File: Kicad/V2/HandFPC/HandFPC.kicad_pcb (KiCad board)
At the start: 2 copper layers, 25 parts, among them J10 SPI_LED, J2 JST_LED_SPI_5V_GND, J3 JST_LED_SPI_5V_GND, J4 JST_LED_SPI_5V_GND, J5 JST_LED_SPI_5V_GND, J6 JST_LED_SPI_5V_GND, J7 SPI_LED, J8 SPI_LED, J9 SPI_LED, U1 ICM-42688-P_I2C, U2 Hall Sensor DRV5023

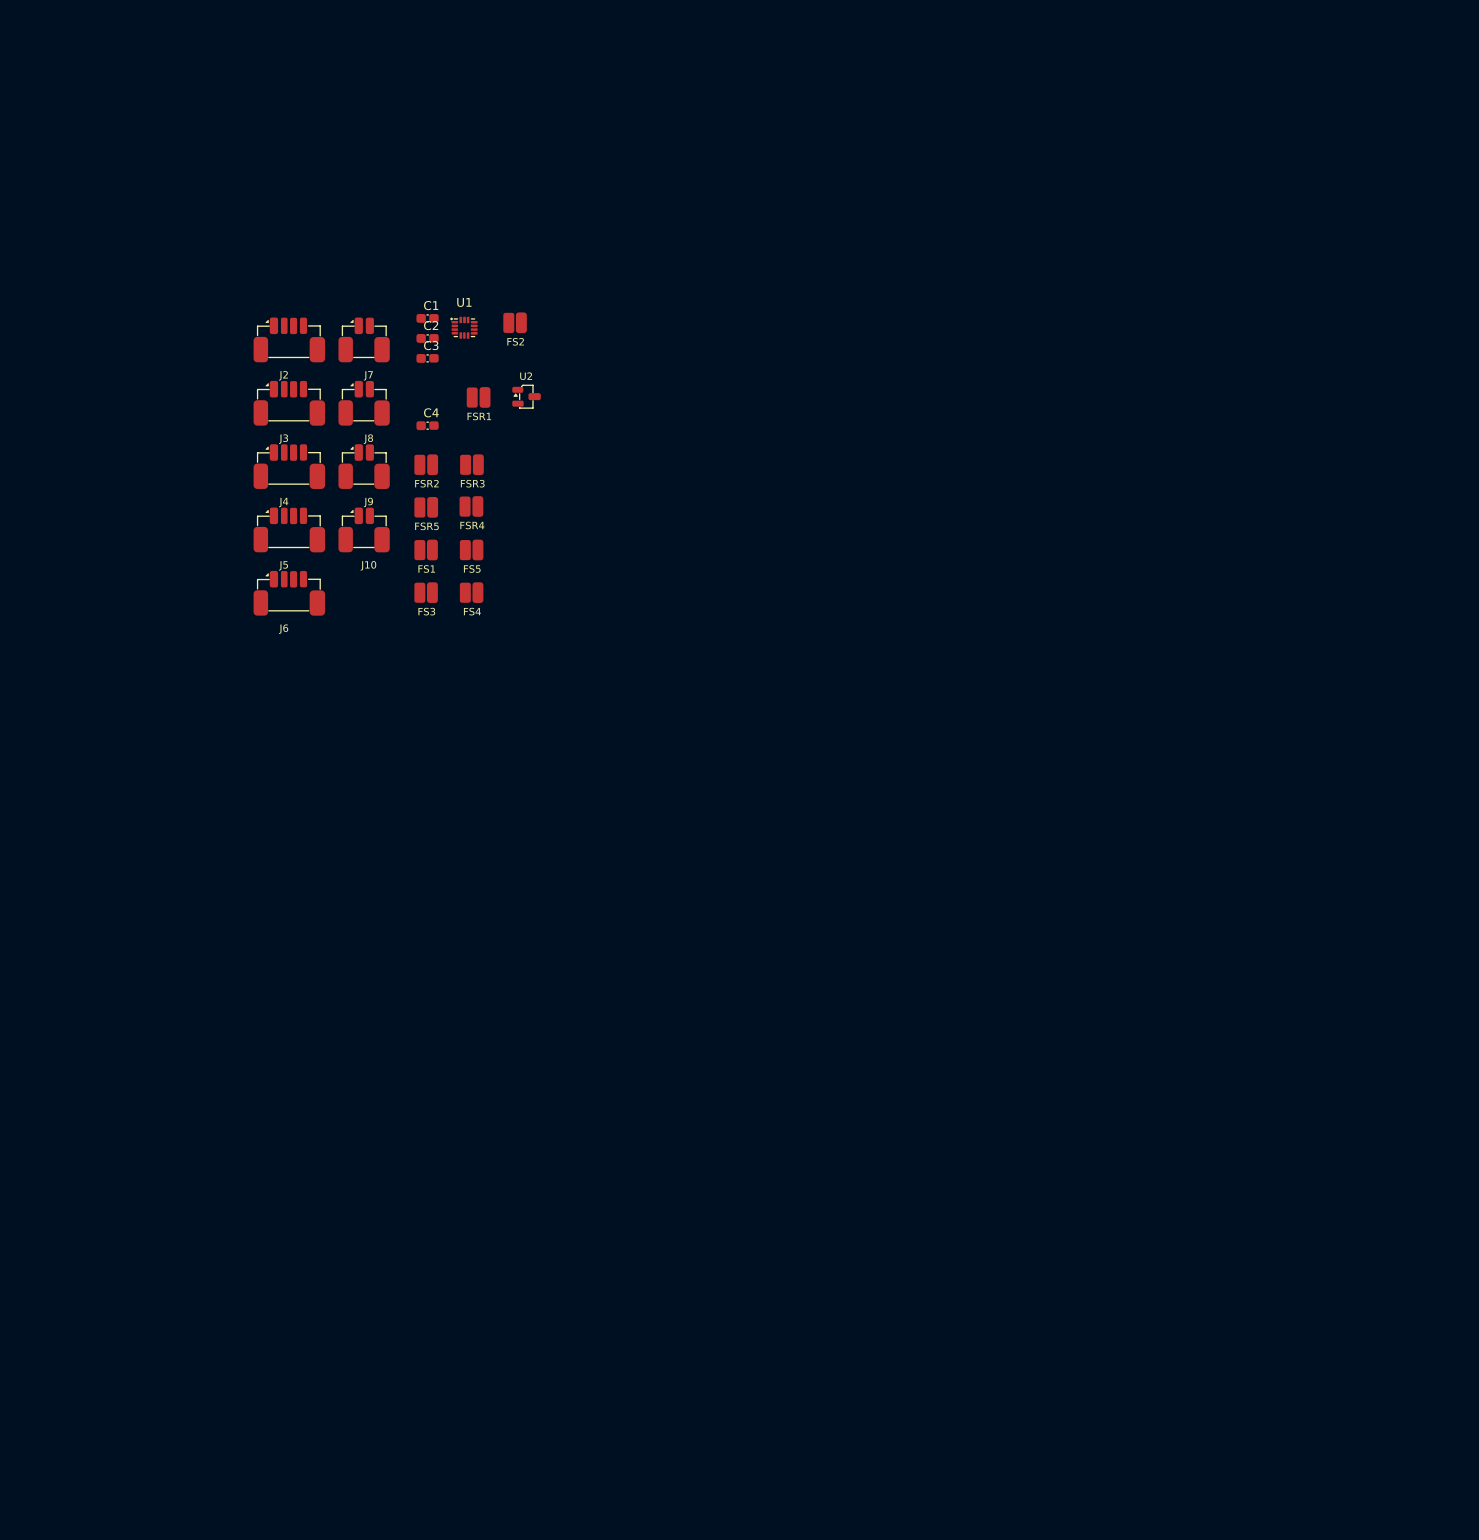
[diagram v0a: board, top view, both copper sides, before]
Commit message: add edgecut for testing
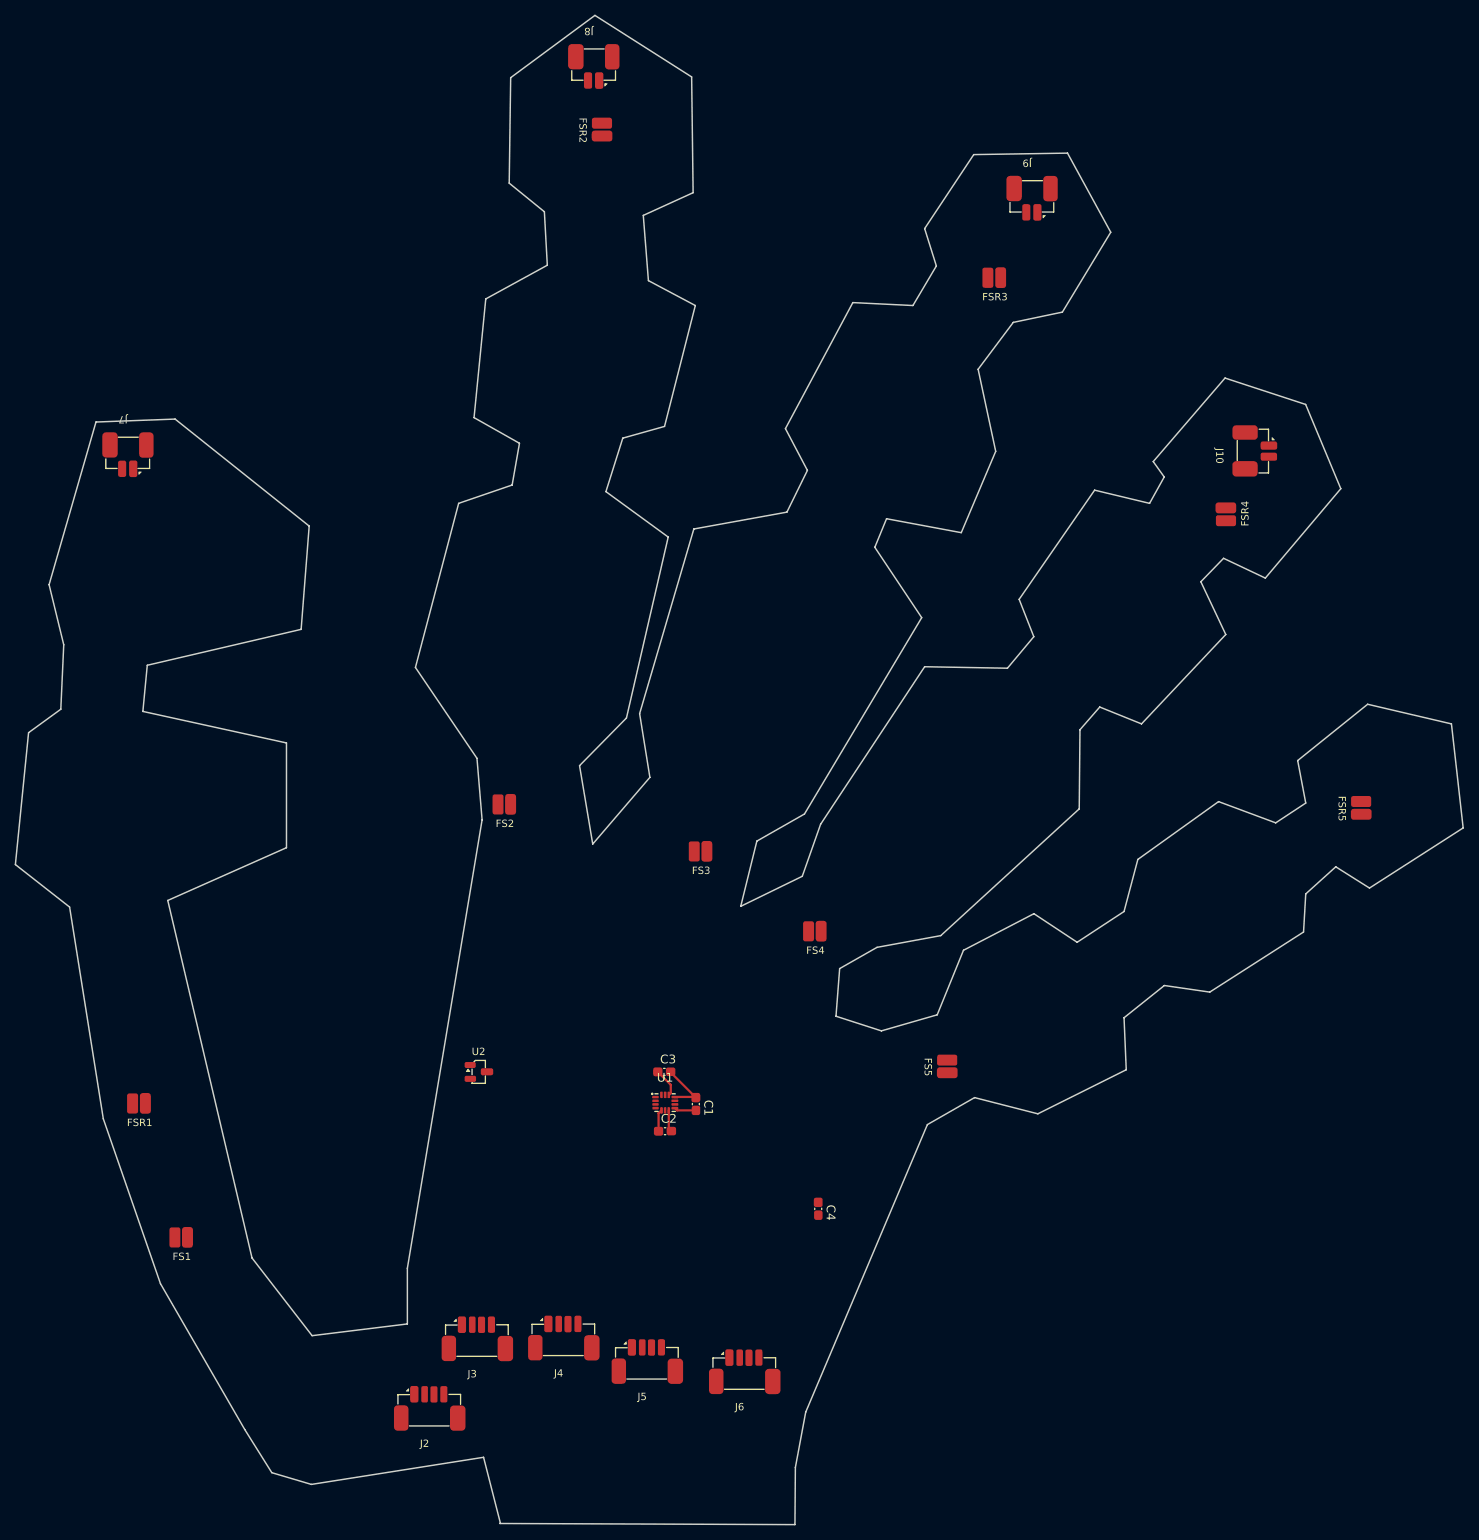
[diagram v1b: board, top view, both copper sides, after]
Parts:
- moved J2 147.1 mm to (52.3, 183.0)
- moved FSR5 134.0 mm to (184.3, 97.4), turned to -90 degrees
- moved J3 130.2 mm to (58.8, 173.5)
- moved J4 124.7 mm to (70.6, 173.4)
- moved J5 123.6 mm to (82.0, 176.6)
- moved J6 123.1 mm to (95.3, 178.0)
- moved J10 122.8 mm to (166.1, 45.1), turned to -90 degrees
- moved C4 119.4 mm to (110.2, 152.1), turned to -90 degrees
- moved C1 113.3 mm to (93.5, 137.8), turned to -90 degrees
- moved C2 113.0 mm to (89.3, 141.5)
- moved U1 109.2 mm to (89.3, 137.6)
- moved J9 107.6 mm to (142.9, 10.5), turned to 180 degrees
- moved FSR1 106.9 mm to (17.5, 137.7)
- moved FSR4 103.0 mm to (165.8, 57.3), turned to 90 degrees
- moved C3 102.6 mm to (89.2, 133.4)
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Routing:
- net GND: track 0.00 -> 10.8 mm
- net +3.3V: track 0.00 -> 9.96 mm
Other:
- board outline added: 197.6 x 206 mm
